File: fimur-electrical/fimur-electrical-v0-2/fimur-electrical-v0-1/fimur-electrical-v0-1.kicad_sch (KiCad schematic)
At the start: 14 parts, among them J1 Conn_01x04_Pin, J2 Conn_01x04_Pin, J3 Conn_02x03_Odd_Even, U1 NCP163AFCS180T2G, U2 ICM-20948, U3 ICM-20948

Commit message: multiplex schematic and layout and standardization with 2-imu board
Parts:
- J1, J2: footprint Connector_JST:JST_PH_B4B-PH-K_1x04_P2.00mm_Vertical -> Connector_JST:JST_SH_SM04B-SRSS-TB_1x04-1MP_P1.00mm_Horizontal
- J3: footprint Connector_PinSocket_2.54mm:PinSocket_2x03_P2.54mm_Vertical -> Connector_PinSocket_2.54mm:PinSocket_2x03_P2.54mm_Horizontal
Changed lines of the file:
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@@
 			)
 		)
-		(property "Footprint" "Connector_PinSocket_2.54mm:PinSocket_2x03_P2.54mm_Vertical"
+		(property "Footprint" "Connector_PinSocket_2.54mm:PinSocket_2x03_P2.54mm_Horizontal"
 			(at 86.36 106.68 0)
 			(effects
@@
 			)
 		)
-		(property "Footprint" "Connector_JST:JST_PH_B4B-PH-K_1x04_P2.00mm_Vertical"
+		(property "Footprint" "Connector_JST:JST_SH_SM04B-SRSS-TB_1x04-1MP_P1.00mm_Horizontal"
 			(at 20.32 105.41 0)
 			(effects
@@
 			)
 		)
-		(property "Footprint" "Connector_JST:JST_PH_B4B-PH-K_1x04_P2.00mm_Vertical"
+		(property "Footprint" "Connector_JST:JST_SH_SM04B-SRSS-TB_1x04-1MP_P1.00mm_Horizontal"
 			(at 20.32 90.17 0)
 			(effects

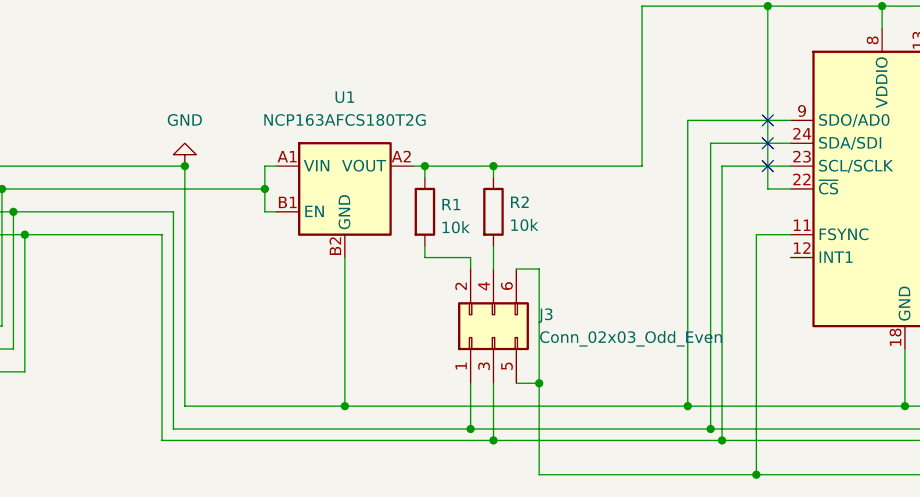
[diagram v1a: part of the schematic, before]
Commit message: cleanup of v10.1.1
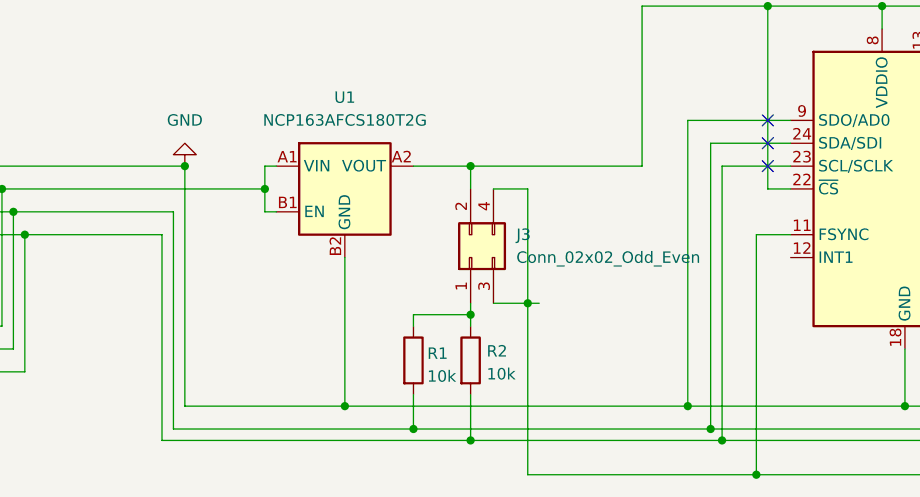
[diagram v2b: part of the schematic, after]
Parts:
- removed J3: Conn_02x03_Odd_Even, Connector_PinSocket_2.54mm:PinSocket_2x03_P2.54mm_Horizontal, symbol Connector_Generic:Conn_02x03_Odd_Even
- added J3: Conn_02x02_Odd_Even, Connector_PinSocket_2.54mm:PinSocket_2x02_P2.54mm_Horizontal, symbol Connector_Generic:Conn_02x02_Odd_Even
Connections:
- net at C2.1, C3.1, C5.1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: now also J3.2 (Pin_2); no longer R1.1, R2.1
- net at J1.3 (Pin_3), J2.3 (Pin_3), U2.24 (SDA/SDI)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: now also R1.2
- net at J1.4 (Pin_4), J2.4 (Pin_4), U2.23 (SCL/SCLK)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: now also R2.2
- net at U2.11 (FSYNC), U3.11 (FSYNC): now also J3.3 (Pin_3), J3.4 (Pin_4)
- new net: J3.1 (Pin_1), R1.1, R2.1
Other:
- moved on the sheet: R1, R2
